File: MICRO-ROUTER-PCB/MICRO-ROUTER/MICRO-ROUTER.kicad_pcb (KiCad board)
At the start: 2 copper layers, 85 x 54 mm, 77 parts, among them J2 USB_A, J3 USB_C_Receptacle_USB2.0_16P, J4 Battery Connector, J5 SPI Header, J6 GPIO Header, J7 RJ45 5-2301996-6, Q1 FS8205A, SW2 8Devices Reset, SW3 UART Reset, U1 TP4056, U2 XC9142B33DMR-G, U3 CP2102N-Axx-xQFN20, U4 DW01A, U5 XC9141A50DMR-G, X1 142-0711-821

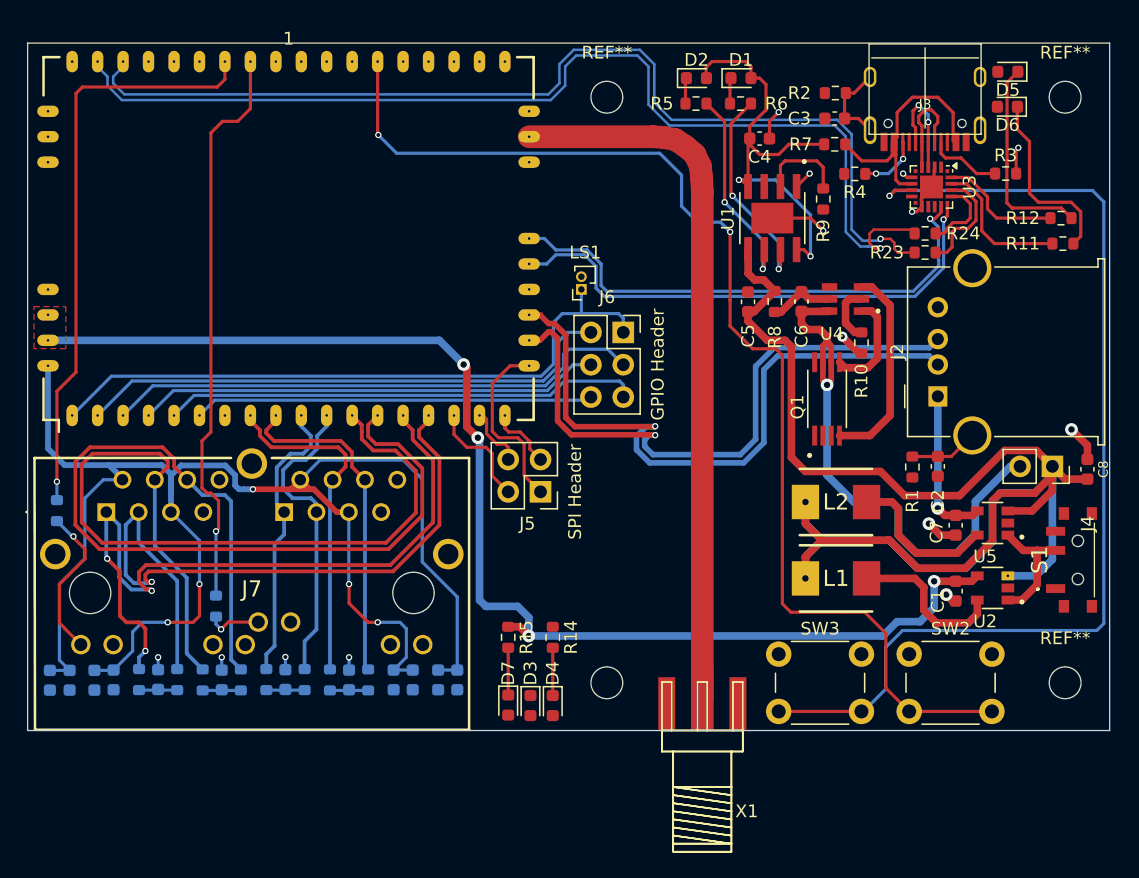
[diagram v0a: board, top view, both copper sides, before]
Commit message: finished layout
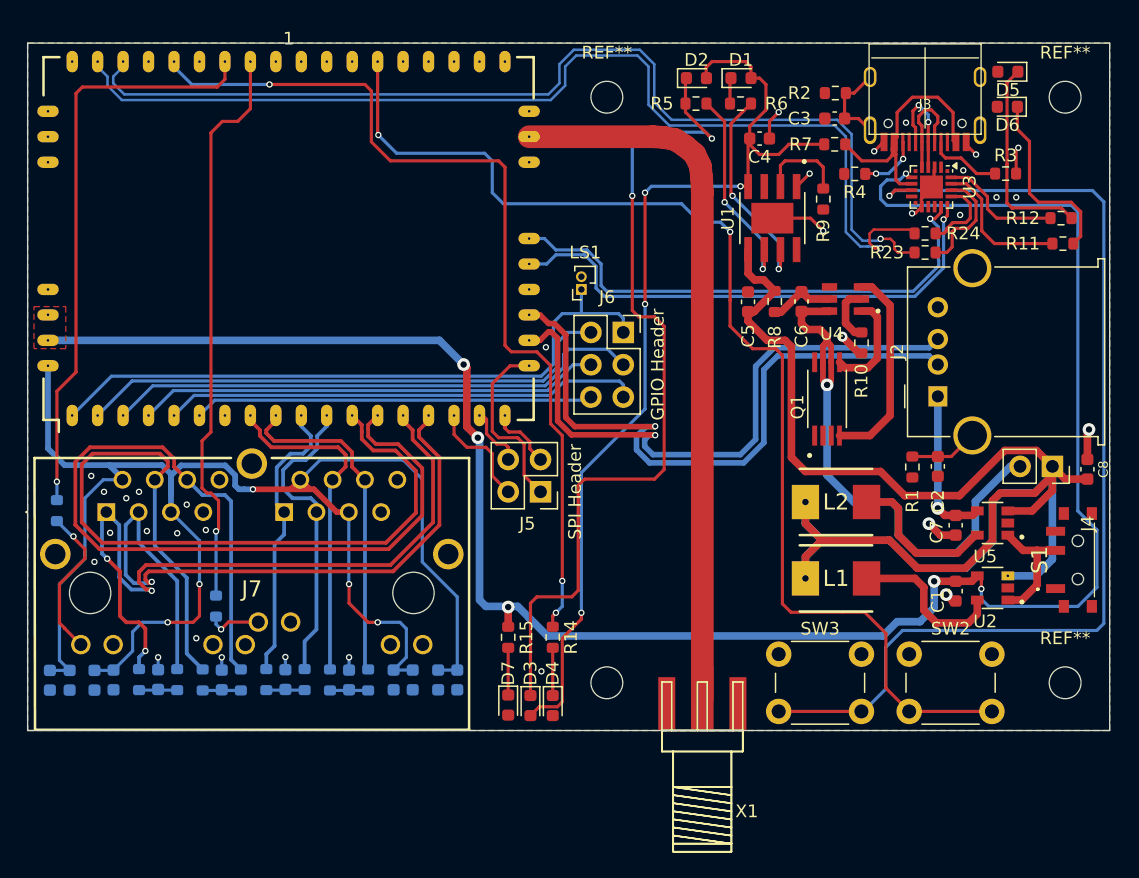
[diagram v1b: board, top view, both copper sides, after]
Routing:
- net Net-(1-LED0): track 0.00 -> 71.5 mm, vias 0 -> 3
- net Net-(D2-K): track 2.03 -> 67.0 mm, vias 0 -> 2
- net +3.3V: track 99.5 -> 159.5 mm, vias 5 -> 6
- net Net-(D1-A): track 34.9 -> 76.6 mm, vias 2 -> 4
- net GND: track 27.2 -> 29.1 mm, vias 13 -> 34
- added copper zone on B.Cu, net GND
- added copper zone on F.Cu, net GND
